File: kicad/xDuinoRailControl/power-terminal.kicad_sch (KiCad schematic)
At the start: 5 parts, among them J2 Screw_Terminal_01x02, U1 DRV8870DDA

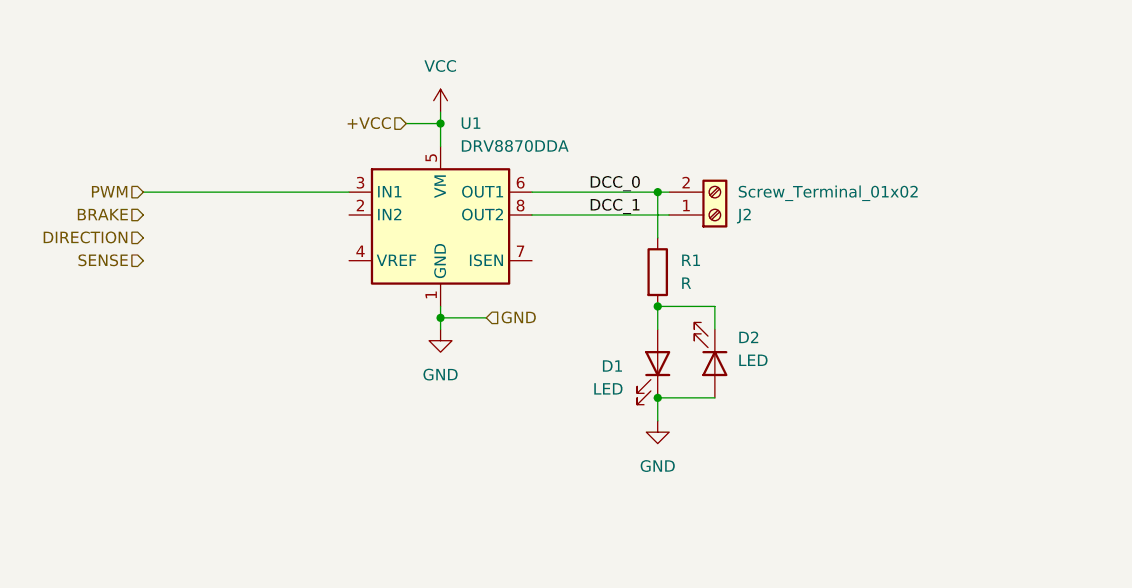
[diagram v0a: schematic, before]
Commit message: xDuinoRailControl
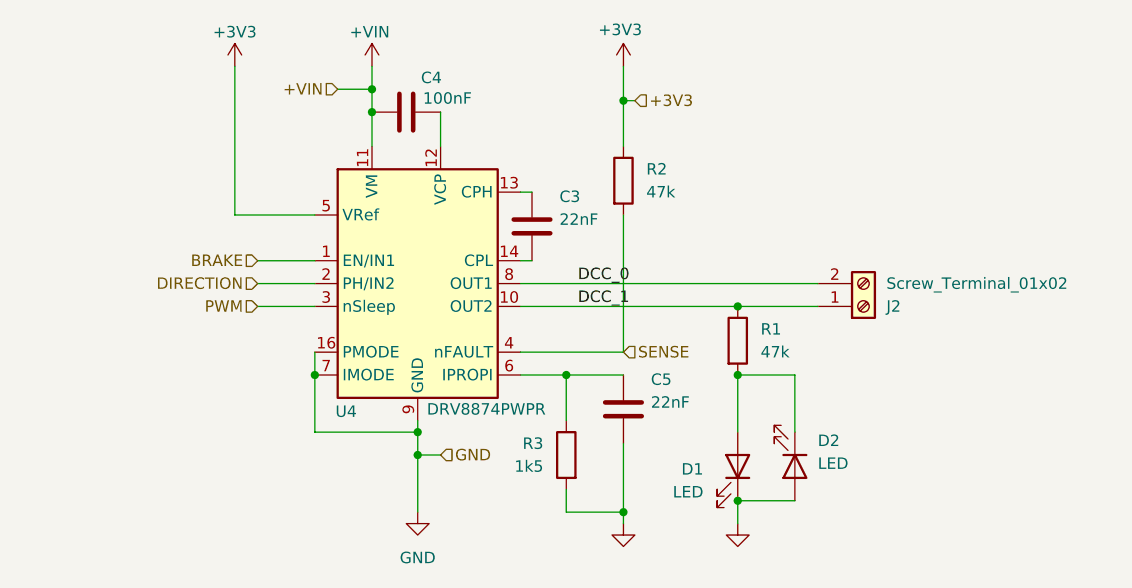
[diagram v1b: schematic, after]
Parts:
- removed U1: DRV8870DDA, Package_SO:Texas_HTSOP-8-1EP_3.9x4.9mm_P1.27mm_EP2.95x4.9mm_Mask2.4x3.1mm_ThermalVias, symbol Driver_Motor:DRV8870DDA
- added C3, C5: 22nF, Capacitor_SMD:C_0805_2012Metric_Pad1.18x1.45mm_HandSolder, symbol Device:C
- added C4: 100nF, Capacitor_SMD:C_0805_2012Metric_Pad1.18x1.45mm_HandSolder, symbol Device:C
- added R2: 47k, Resistor_SMD:R_0805_2012Metric_Pad1.20x1.40mm_HandSolder, symbol Device:R
- added R3: 1k5, Resistor_SMD:R_0805_2012Metric_Pad1.20x1.40mm_HandSolder, symbol Device:R
- added U4: DRV8874PWPR, DRVC8874:HTSSOP-16-1EP_4.4x5mm_P0.65mm_EP3.4x5mm_Mask2.46_HiAmp, symbol _my:DRV8874PWPR
- D1, D2: LCSC (none) -> C2296
- J2: LCSC (none) -> C784937
- R1: value R -> 47k; LCSC (none) -> C17713
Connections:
- net BRAKE: now also U4.1 (EN/IN1)
- net DCC_0: now also U4.8 (OUT1); no longer R1.1
- net DCC_1: now also R1.1, U4.10 (OUT2)
- net DIRECTION: now also U4.2 (PH/IN2)
- net GND: now also C5.2, R3.2, U4.15 (GND), U4.16 (PMODE), U4.17 (GND), U4.7 (IMODE), U4.9 (GND)
- net PWM: now also U4.3 (nSleep)
- net SENSE: now also R2.2, U4.4 (nFAULT)
- new net: C5.1, R3.1, U4.6 (IPROPI)
- new net: C4.1, U4.12 (VCP)
- new net: C3.1, U4.13 (CPH)
- new net: C3.2, U4.14 (CPL)
- new net +3V3: R2.1, U4.5 (VRef)
- new net +VIN: C4.2, U4.11 (VM)
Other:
- moved on the sheet: D1, D2, J2, R1
